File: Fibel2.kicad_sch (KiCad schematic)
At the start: 0 parts

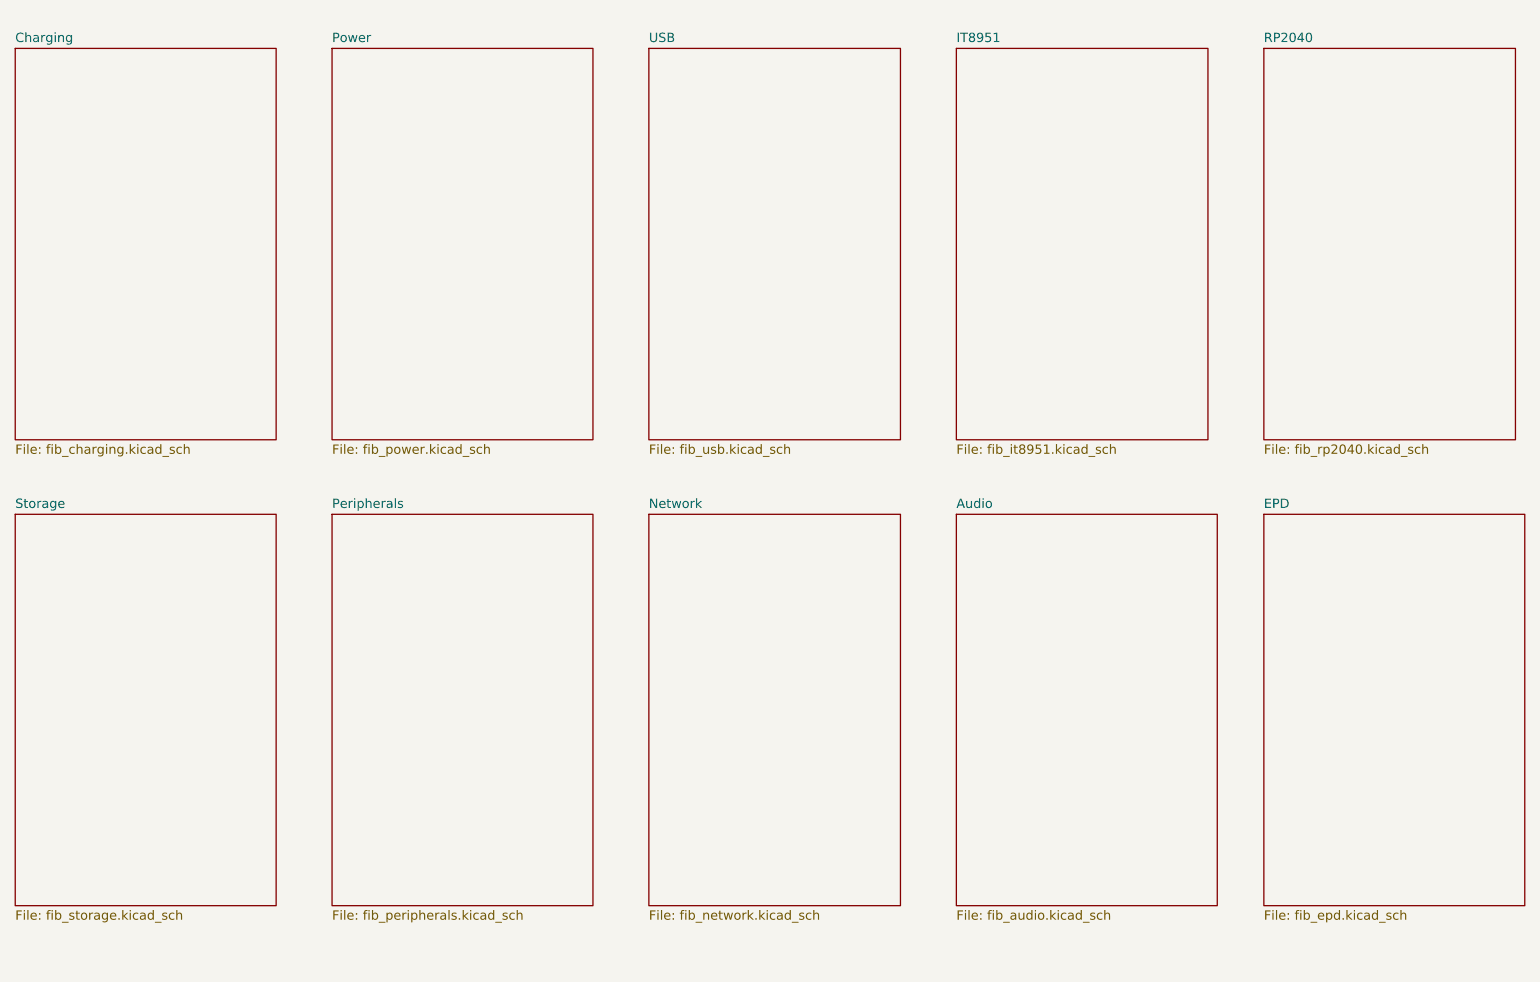
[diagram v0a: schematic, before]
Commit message: added symbol&footprint for orin/sodimm, added a bunch of specs and docs, partially implemented audio, full steam ahead
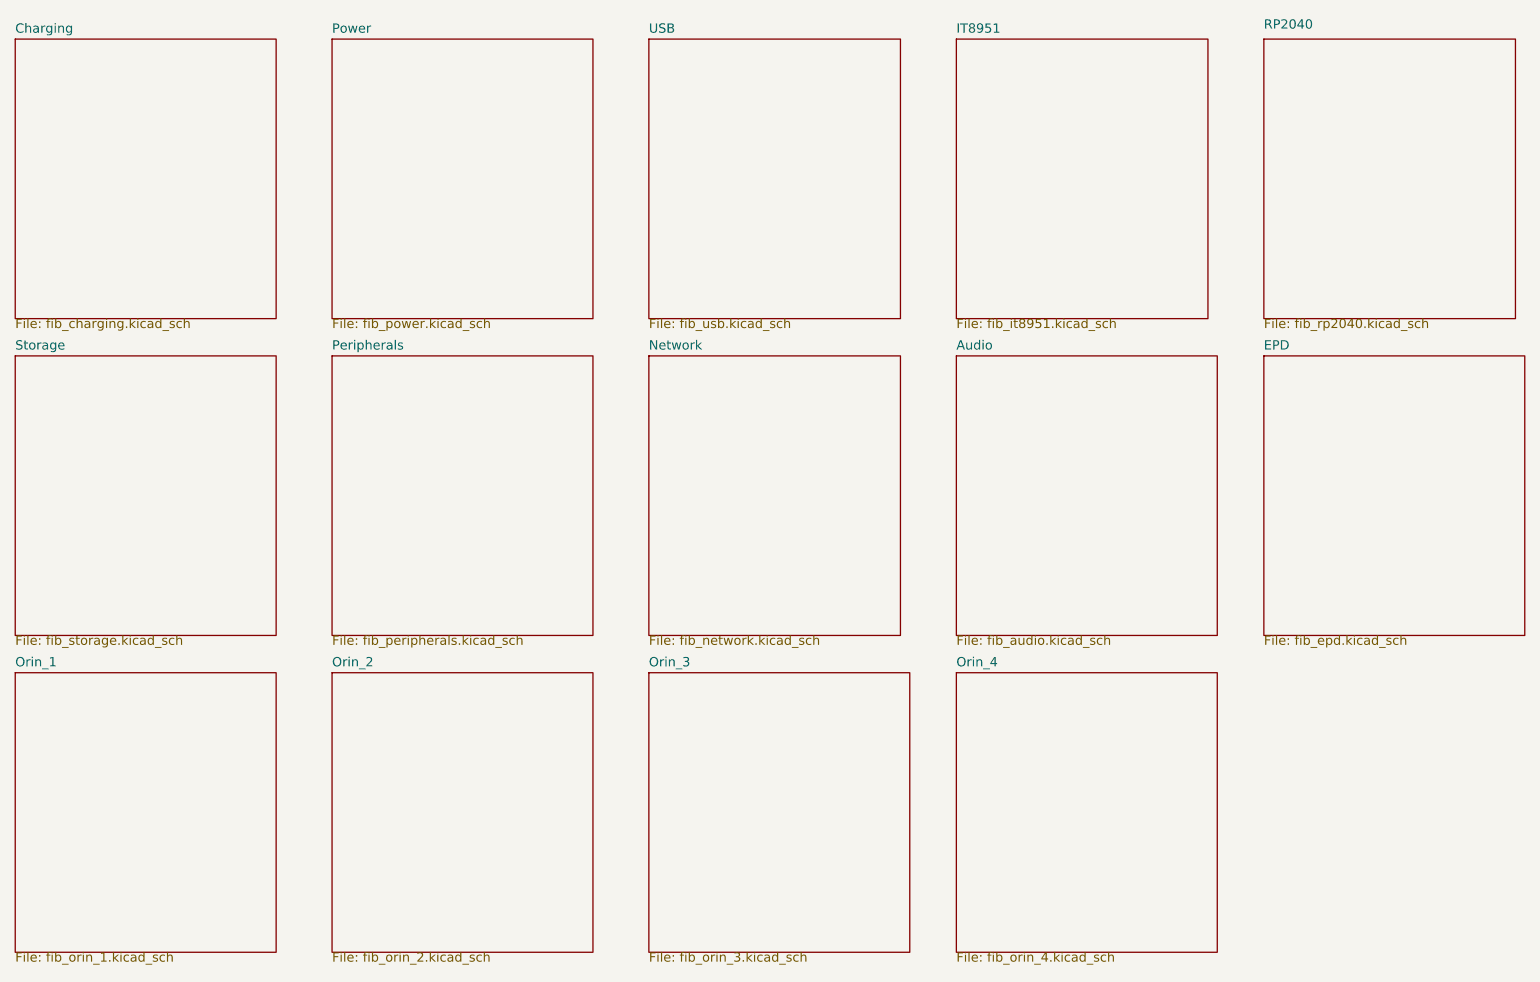
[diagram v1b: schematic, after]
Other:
- added sheet Orin_1 (fib_orin_1.kicad_sch)
- added sheet Orin_2 (fib_orin_2.kicad_sch)
- added sheet Orin_3 (fib_orin_3.kicad_sch)
- added sheet Orin_4 (fib_orin_4.kicad_sch)
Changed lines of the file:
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@@
 	(paper "A4")
 	(sheet
-		(at 154.94 85.09)
-		(size 35.56 53.34)
+		(at 154.94 63.5)
+		(size 35.56 38.1)
 		(fields_autoplaced yes)
 		(stroke
@@
 		)
 		(property "Sheetname" "Audio"
-			(at 154.94 84.3784 0)
+			(at 154.94 62.7884 0)
 			(effects
 				(font
@@
 		)
 		(property "Sheetfile" "fib_audio.kicad_sch"
-			(at 154.94 139.0146 0)
+			(at 154.94 101.5496 0)
 			(effects
 				(font
@@
 	)
 	(sheet
-		(at 26.67 21.59)
-		(size 35.56 53.34)
+		(at 26.67 20.32)
+		(size 35.56 38.1)
 		(fields_autoplaced yes)
 		(stroke
@@
 		)
 		(property "Sheetname" "Charging"
-			(at 26.67 20.8784 0)
+			(at 26.67 19.6084 0)
 			(effects
 				(font
@@
 		)
 		(property "Sheetfile" "fib_charging.kicad_sch"
-			(at 26.67 75.5146 0)
+			(at 26.67 58.3696 0)
 			(effects
 				(font
@@
 	)
 	(sheet
-		(at 196.85 21.59)
-		(size 34.29 53.34)
+		(at 196.85 20.32)
+		(size 34.29 38.1)
 		(fields_autoplaced yes)
 		(stroke
@@
 		)
 		(property "Sheetname" "RP2040"
-			(at 196.85 20.8784 0)
+			(at 196.85 19.05 0)
 			(effects
 				(font
@@
 		)
 		(property "Sheetfile" "fib_rp2040.kicad_sch"
-			(at 196.85 75.5146 0)
+			(at 196.85 58.3696 0)
 			(effects
 				(font
@@
 	)
 	(sheet
-		(at 196.85 85.09)
-		(size 35.56 53.34)
+		(at 113.03 106.68)
+		(size 35.56 38.1)
+		(fields_autoplaced yes)
+		(stroke
+			(width 0.1524)
+			(type solid)
+		)
+		(fill
+			(color 0 0 0 0.0000)
+		)
+		(property "Sheetname" "Orin_3"
+			(at 113.03 105.9684 0)
+			(effects
+				(font
+					(size 1.27 1.27)
+				)
+				(justify left bottom)
+			)
+		)
+		(property "Sheetfile" "fib_orin_3.kicad_sch"
+			(at 113.03 144.7296 0)
+			(effects
+				(font
+					(size 1.27 1.27)
+				)
+				(justify left top)
+			)
+		)
+		(instances
+			(project "Fibel2"
+				(path "/862c21e2-7ec9-4f80-a33c-aad02ea9423e"
+					(page "14")
+				)
+			)
+		)
+	)
+	(sheet
+		(at 196.85 63.5)
+		(size 35.56 38.1)
 		(fields_autoplaced yes)
 		(stroke
@@
 		)
 		(property "Sheetname" "EPD"
-			(at 196.85 84.3784 0)
+			(at 196.85 62.7884 0)
 			(effects
 				(font
@@
 		)
 		(property "Sheetfile" "fib_epd.kicad_sch"
-			(at 196.85 139.0146 0)
+			(at 196.85 101.5496 0)
 			(effects
 				(font
@@
 	)
 	(sheet
-		(at 26.67 85.09)
-		(size 35.56 53.34)
+		(at 69.85 106.68)
+		(size 35.56 38.1)
+		(fields_autoplaced yes)
+		(stroke
+			(width 0.1524)
+			(type solid)
+		)
+		(fill
+			(color 0 0 0 0.0000)
+		)
+		(property "Sheetname" "Orin_2"
+			(at 69.85 105.9684 0)
+			(effects
+				(font
+					(size 1.27 1.27)
+				)
+				(justify left bottom)
+			)
+		)
+		(property "Sheetfile" "fib_orin_2.kicad_sch"
+			(at 69.85 144.7296 0)
+			(effects
+				(font
+					(size 1.27 1.27)
+				)
+				(justify left top)
+			)
+		)
+		(instances
+			(project "Fibel2"
+				(path "/862c21e2-7ec9-4f80-a33c-aad02ea9423e"
+					(page "13")
+				)
+			)
+		)
+	)
+	(sheet
+		(at 26.67 63.5)
+		(size 35.56 38.1)
 		(fields_autoplaced yes)
 		(stroke
@@
 		)
 		(property "Sheetname" "Storage"
-			(at 26.67 84.3784 0)
+			(at 26.67 62.7884 0)
 			(effects
 				(font
@@
 		)
 		(property "Sheetfile" "fib_storage.kicad_sch"
-			(at 26.67 139.0146 0)
+			(at 26.67 101.5496 0)
 			(effects
 				(font
@@
 	)
 	(sheet
-		(at 69.85 21.59)
-		(size 35.56 53.34)
+		(at 69.85 20.32)
+		(size 35.56 38.1)
 		(fields_autoplaced yes)
 		(stroke
@@
 		)
 		(property "Sheetname" "Power"
-			(at 69.85 20.8784 0)
+			(at 69.85 19.6084 0)
 			(effects
 				(font
@@
 		)
 		(property "Sheetfile" "fib_power.kicad_sch"
-			(at 69.85 75.5146 0)
+			(at 69.85 58.3696 0)
 			(effects
 				(font
@@
 	)
 	(sheet
-		(at 113.03 21.59)
-		(size 34.29 53.34)
+		(at 113.03 20.32)
+		(size 34.29 38.1)
 		(fields_autoplaced yes)
 		(stroke
@@
 		)
 		(property "Sheetname" "USB"
-			(at 113.03 20.8784 0)
+			(at 113.03 19.6084 0)
 			(effects
 				(font
@@
 		)
 		(property "Sheetfile" "fib_usb.kicad_sch"
-			(at 113.03 75.5146 0)
+			(at 113.03 58.3696 0)
 			(effects
 				(font
@@
 	)
 	(sheet
-		(at 69.85 85.09)
-		(size 35.56 53.34)
+		(at 69.85 63.5)
+		(size 35.56 38.1)
 		(fields_autoplaced yes)
 		(stroke
@@
 		)
 		(property "Sheetname" "Peripherals"
-			(at 69.85 84.3784 0)
+			(at 69.85 62.7884 0)
 			(effects
 				(font
@@
 		)
 		(property "Sheetfile" "fib_peripherals.kicad_sch"
-			(at 69.85 139.0146 0)
+			(at 69.85 101.5496 0)
 			(effects
 				(font
@@
 	)
 	(sheet
-		(at 113.03 85.09)
-		(size 34.29 53.34)
+		(at 113.03 63.5)
+		(size 34.29 38.1)
 		(fields_autoplaced yes)
 		(stroke
@@
 		)
 		(property "Sheetname" "Network"
-			(at 113.03 84.3784 0)
+			(at 113.03 62.7884 0)
 			(effects
 				(font
@@
 		)
 		(property "Sheetfile" "fib_network.kicad_sch"
-			(at 113.03 139.0146 0)
+			(at 113.03 101.5496 0)
 			(effects
 				(font
@@
 	)
 	(sheet
-		(at 154.94 21.59)
-		(size 34.29 53.34)
+		(at 26.67 106.68)
+		(size 35.56 38.1)
+		(fields_autoplaced yes)
+		(stroke
+			(width 0.1524)
+			(type solid)
+		)
+		(fill
+			(color 0 0 0 0.0000)
+		)
+		(property "Sheetname" "Orin_1"
+			(at 26.67 105.9684 0)
+			(effects
+				(font
+					(size 1.27 1.27)
+				)
+				(justify left bottom)
+			)
+		)
+		(property "Sheetfile" "fib_orin_1.kicad_sch"
+			(at 26.67 144.7296 0)
+			(effects
+				(font
+					(size 1.27 1.27)
+				)
+				(justify left top)
+			)
+		)
+		(instances
+			(project "Fibel2"
+				(path "/862c21e2-7ec9-4f80-a33c-aad02ea9423e"
+					(page "12")
+				)
+			)
+		)
+	)
+	(sheet
+		(at 154.94 106.68)
+		(size 35.56 38.1)
+		(fields_autoplaced yes)
+		(stroke
+			(width 0.1524)
+			(type solid)
+		)
+		(fill
+			(color 0 0 0 0.0000)
+		)
+		(property "Sheetname" "Orin_4"
+			(at 154.94 105.9684 0)
+			(effects
+				(font
+					(size 1.27 1.27)
+				)
+				(justify left bottom)
+			)
+		)
+		(property "Sheetfile" "fib_orin_4.kicad_sch"
+			(at 154.94 144.7296 0)
+			(effects
+				(font
+					(size 1.27 1.27)
+				)
+				(justify left top)
+			)
+		)
+		(instances
+			(project "Fibel2"
+				(path "/862c21e2-7ec9-4f80-a33c-aad02ea9423e"
+					(page "15")
+				)
+			)
+		)
+	)
+	(sheet
+		(at 154.94 20.32)
+		(size 34.29 38.1)
 		(fields_autoplaced yes)
 		(stroke
@@
 		)
 		(property "Sheetname" "IT8951"
-			(at 154.94 20.8784 0)
+			(at 154.94 19.6084 0)
 			(effects
 				(font
@@
 		)
 		(property "Sheetfile" "fib_it8951.kicad_sch"
-			(at 154.94 75.5146 0)
-			(effects
-				(font
+			(at 154.94 58.3696 0)
+			(effects
+				(font
